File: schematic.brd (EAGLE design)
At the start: 37.8 x 60.9 mm, 17 parts, among them IC1 TL071P, IC2 ATTINY402-SSF, IC3 7805T, X1 PG203J

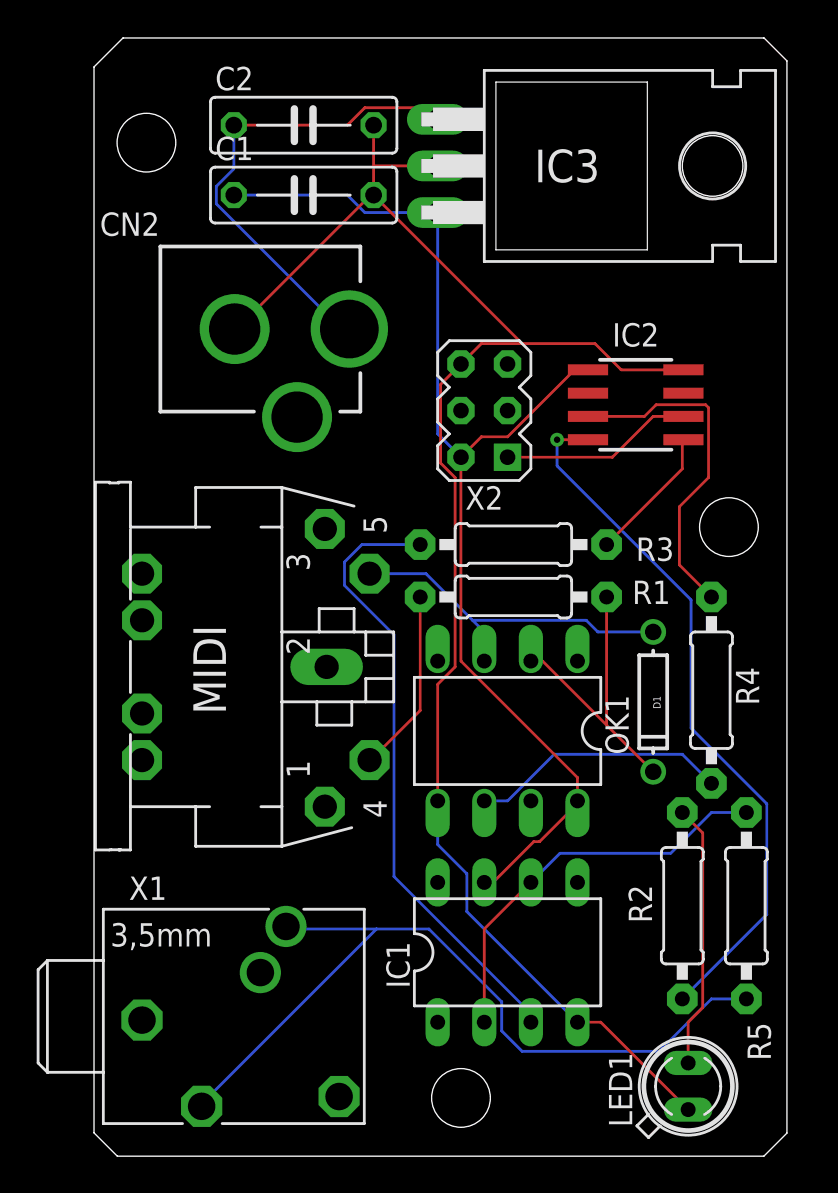
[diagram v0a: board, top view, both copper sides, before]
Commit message: Restructured Project
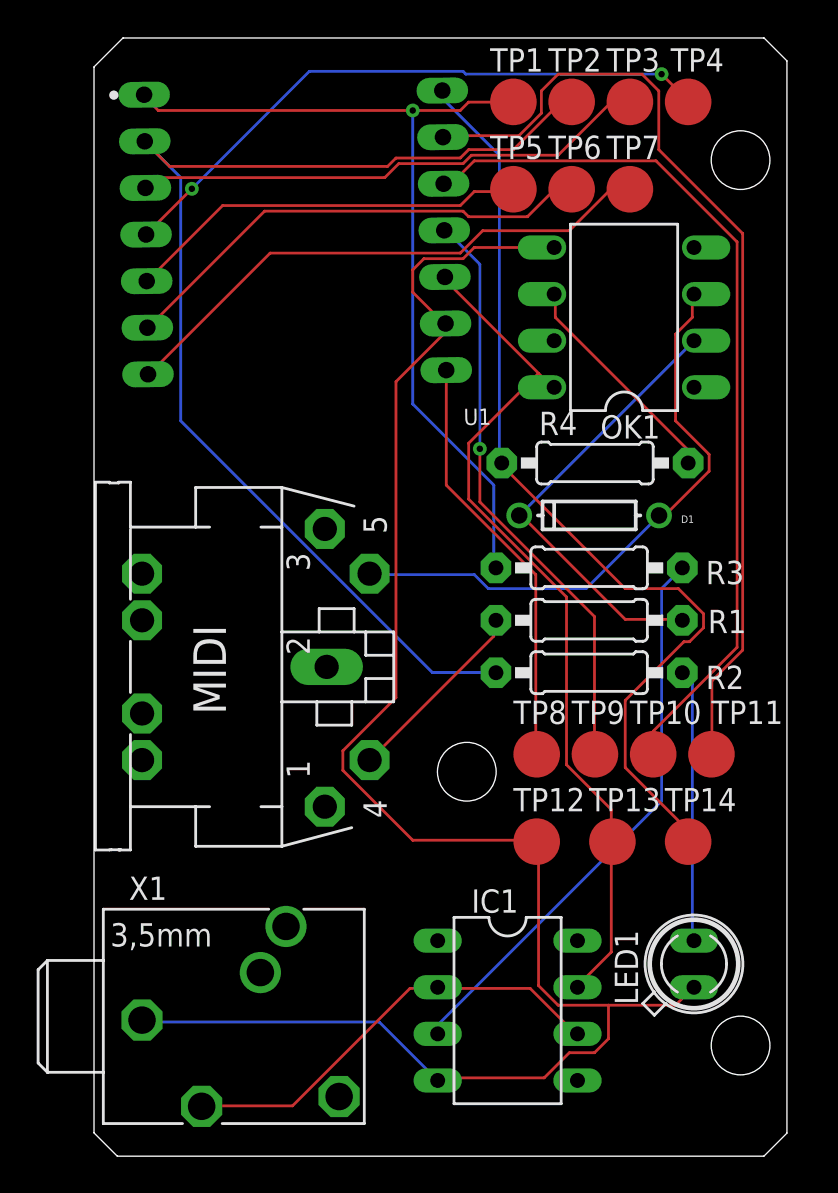
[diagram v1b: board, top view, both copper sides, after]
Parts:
- removed C1: 0.1u, rcl:C075-032X103
- removed C2: 0.33u, rcl:C075-032X103
- removed CN2: (no value), adafruit:DCJACK_2MM_PTH
- removed IC2: ATTINY402-SSF, atmel:SO8
- removed IC3: 7805T, adafruit:TO220H
- removed R5: 470, adafruit:0207/10
- removed X2: (no value), atmel:PINHEADER_2R03_100MIL
- added TP1, TP10, TP11, TP12, TP13, TP14, TP2, TP3, TP4, TP5, TP6, TP7, TP8, TP9: TPB2,54, testpad:B2,54
- added U1: (no value), Seeeduino XIAO_holes:MOUDLE14P-2.54-21X17.8MM
- moved OK1 23.4 mm to (28.9, 61.0), turned to 90 degrees
- moved R4 13.9 mm to (27.3, 53.0), turned to 0 degrees
- moved R2 13.7 mm to (27.0, 41.6), turned to 180 degrees
- moved D1 10.7 mm to (27.0, 50.2), turned to 180 degrees
- moved LED1 6.68 mm to (32.7, 25.7)
- moved R3 4.32 mm to (27.0, 47.3)
- moved R1 4.32 mm to (27.0, 44.5)
- moved IC1 3.18 mm to (22.5, 23.2), turned to 270 degrees
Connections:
- removed net GND: C1.2, C2.2, CN2.GND, IC1.4, IC2.8, IC3.2, LED1.K, OK1.5, X2.6
- removed net GNDBREAK: CN2.GNDBREAK
- removed net N$14 (its old number): R5.1, X1.2, X1.5
- removed net VCC: C1.1, IC1.7, IC2.1, IC3.3, OK1.8, X2.2
- new net N$15: IC1.4, LED1.K, OK1.5, TP12.TP, U1.PAD19, X1.1
- new net N$16: R2.2, TP2.TP, U1.PAD1
- new net N$17: TP8.TP, U1.PAD20
- new net N$18: TP9.TP, U1.PAD17
- new net N$19: TP10.TP, U1.PAD16
- new net N$20: TP11.TP, U1.PAD15
- new net N$21: OK1.6, R4.2
- new net N$4: TP3.TP, U1.PAD2
- net N$10: now also R3.1; no longer R3.2
- net N$11: now also X1.5; no longer R5.2
- net N$12: now also TP6.TP, U1.PAD5; no longer IC2.4, R2.2
- net N$13: now also TP7.TP, U1.PAD6; no longer C2.1, CN2.PWR, IC3.1
- net N$5: now also IC1.7, OK1.8, TP13.TP, U1.PAD18; no longer IC2.6, X2.1
- net N$6: now also TP14.TP, U1.PAD14; no longer OK1.6
- net N$7: now also TP4.TP, U1.PAD3; no longer IC2.5, R3.1
- net N$8: now also R3.2, TP1.TP, U1.PAD0; no longer IC2.3, R4.2
- net N$9: now also TP5.TP, U1.PAD4; no longer X1.1
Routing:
- net N$15: track 0.00 -> 97.6 mm
- net GND: track 91.0 -> 0.00 mm
- net N$16: track 0.00 -> 64.2 mm
- net VCC: track 62.6 -> 0.00 mm
- net N$20: track 0.00 -> 53.1 mm
- net N$19: track 0.00 -> 48.2 mm
- net N$14 (its old number): track 43.7 -> 0.00 mm
- net N$6: track 14.1 -> 52.0 mm
- net N$5: track 10.5 -> 47.7 mm
- net N$18: track 0.00 -> 32.0 mm, vias 0 -> 1
- net N$8: track 18.6 -> 47.5 mm, vias 0 -> 1
- net N$4: track 0.00 -> 28.3 mm
- net N$7: track 7.48 -> 33.9 mm, vias 0 -> 2
- net N$17: track 0.00 -> 23.0 mm
- net N$9: track 0.00 -> 22.1 mm
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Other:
- board text added: "Designed by T. Findlay, v1.4"
- board text removed: "Designed by T. Findlay, v1.4_LC"
